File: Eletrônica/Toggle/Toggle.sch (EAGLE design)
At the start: 15 parts, among them Q1 IRLML5203, Q2 MOSFET-NCHANNELBSS123LT1G

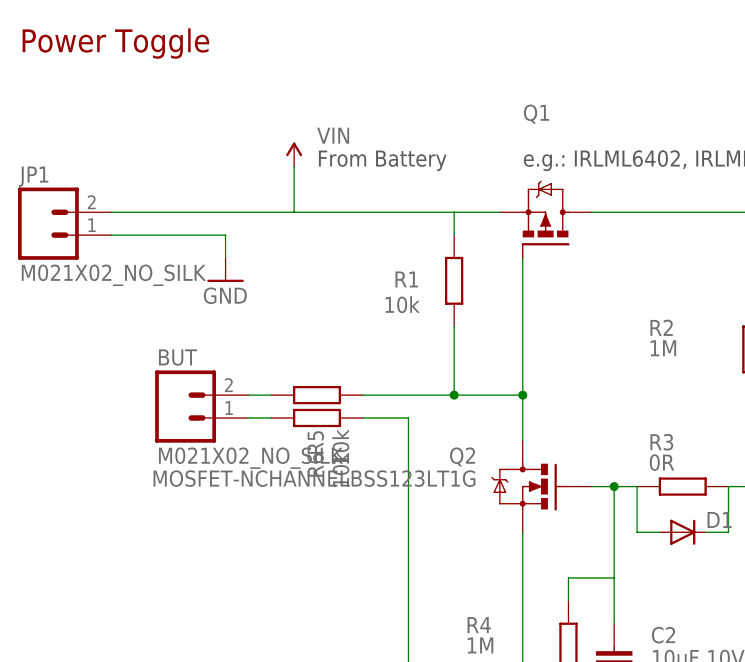
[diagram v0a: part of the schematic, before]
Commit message: Toggle updated
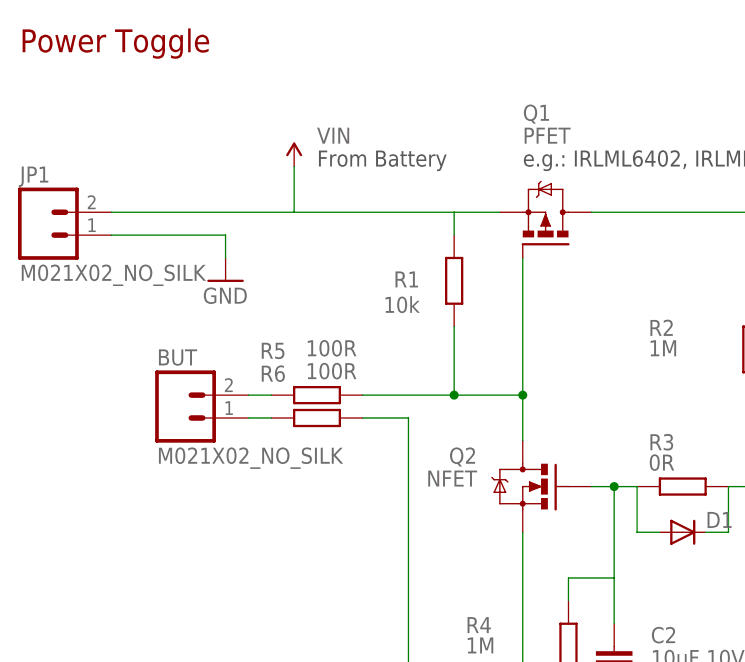
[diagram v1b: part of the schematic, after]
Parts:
- Q1: value IRLML5203 -> PFET
- Q2: value MOSFET-NCHANNELBSS123LT1G -> NFET
- R5, R6: value 10k -> 100R
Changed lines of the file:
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@@
 <parts>
 <part name="R1" library="wes" deviceset="R-EU_" device="R0603" value="10k"/>
-<part name="Q1" library="transistor-power" deviceset="IRLML5203" device="" value=""/>
+<part name="Q1" library="transistor-power" deviceset="IRLML5203" device="" value="PFET"/>
 <part name="R2" library="wes" deviceset="R-EU_" device="R0603" value="1M"/>
 <part name="SUPPLY1" library="SparkFun-Aesthetics" deviceset="VIN" device=""/>
@@
 <part name="C2" library="wes" deviceset="C-EU" device="C0805" value="10uF 10V"/>
 <part name="R3" library="wes" deviceset="R-EU_" device="R0603" value="0R"/>
-<part name="Q2" library="SparkFun-DiscreteSemi" deviceset="MOSFET-NCHANNEL" device="BSS123LT1G" value="MOSFET-NCHANNELBSS123LT1G"/>
+<part name="Q2" library="SparkFun-DiscreteSemi" deviceset="MOSFET-NCHANNEL" device="BSS123LT1G" value="NFET"/>
 <part name="JP1" library="SparkFun-Connectors" deviceset="M02" device="1X02_NO_SILK" value="M021X02_NO_SILK"/>
 <part name="JP3" library="SparkFun-Connectors" deviceset="M03" device="1X03_NO_SILK"/>
 <part name="BUT" library="SparkFun-Connectors" deviceset="M02" device="1X02_NO_SILK" value="M021X02_NO_SILK"/>
-<part name="R5" library="wes" deviceset="R-EU_" device="R0603" value="10k"/>
-<part name="R6" library="wes" deviceset="R-EU_" device="R0603" value="10k"/>
+<part name="R5" library="wes" deviceset="R-EU_" device="R0603" value="100R"/>
+<part name="R6" library="wes" deviceset="R-EU_" device="R0603" value="100R"/>
 <part name="D1" library="SparkFun-DiscreteSemi" deviceset="DIODE" device="SOD523"/>
 <part name="R4" library="wes" deviceset="R-EU_" device="R0603" value="1M"/>
@@
 <instance part="BUT" gate="G$1" x="25.4" y="38.1"/>
 <instance part="R5" gate="G$1" x="40.64" y="40.64" smashed="yes" rot="R180">
-<attribute name="NAME" x="39.5986" y="36.83" size="1.778" layer="95" rot="R270"/>
-<attribute name="VALUE" x="42.418" y="36.83" size="1.778" layer="96" rot="R270"/>
+<attribute name="NAME" x="34.29" y="44.6786" size="1.778" layer="95"/>
+<attribute name="VALUE" x="39.37" y="44.958" size="1.778" layer="96"/>
 </instance>
 <instance part="R6" gate="G$1" x="40.64" y="38.1" smashed="yes" rot="R180">
-<attribute name="NAME" x="39.5986" y="34.29" size="1.778" layer="95" rot="R270"/>
-<attribute name="VALUE" x="42.418" y="34.29" size="1.778" layer="96" rot="R270"/>
+<attribute name="NAME" x="34.29" y="42.1386" size="1.778" layer="95"/>
+<attribute name="VALUE" x="39.37" y="42.418" size="1.778" layer="96"/>
 </instance>
 <instance part="D1" gate="G$1" x="81.28" y="25.4"/>
